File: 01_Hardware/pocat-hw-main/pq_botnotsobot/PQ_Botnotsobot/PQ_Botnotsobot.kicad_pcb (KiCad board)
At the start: 2 copper layers, 64 x 58 mm, 16 parts, among them J1 D2FLA, J2 D2FLA1

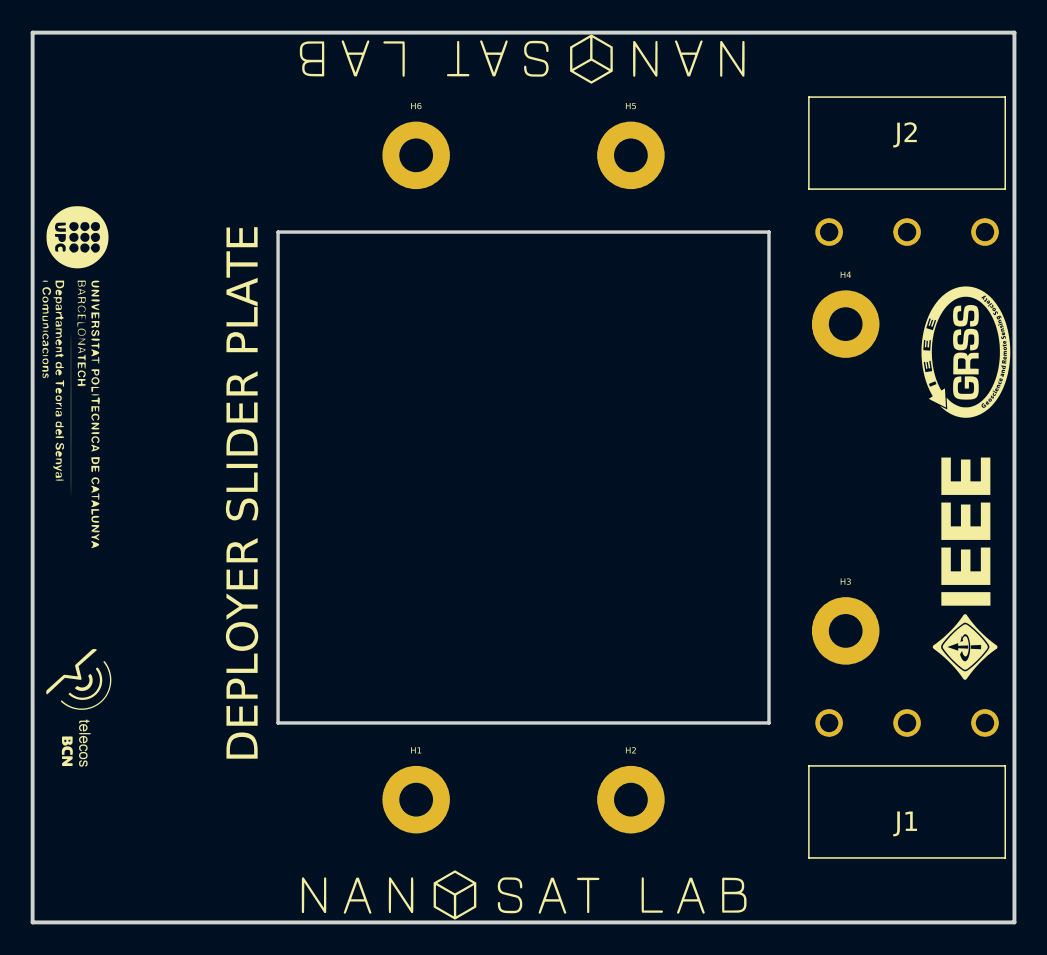
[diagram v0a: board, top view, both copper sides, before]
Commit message: Pcbs actualizados corregidos (son definitivos para mandarlos a fabricar con sus respectivos Gebers en una carpeta separada)
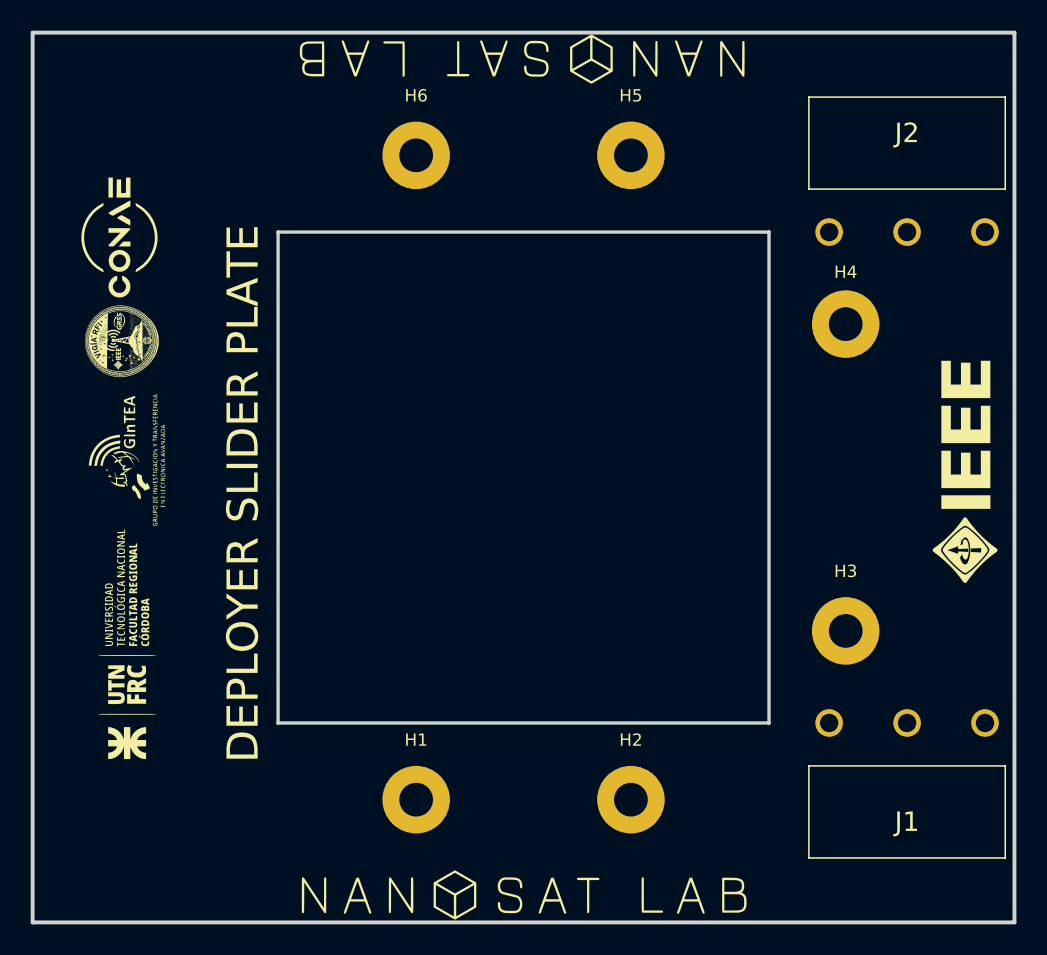
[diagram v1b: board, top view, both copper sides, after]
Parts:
- removed Annotation5: Silkscreen_Annotation, symbols-nsl:GRSS
- removed Annotation8: Silkscreen_Annotation, -nsl_symbols:UPC_positiu
- removed Annotation9: Silkscreen_Annotation, -nsl_symbols:Telecos
- added G***: LOGO, LOGO, F.Cu at (76.5, 53.4)
- added G***: LOGO, LOGO, F.Cu at (76.7, 61.1)
- added G***: LOGO, LOGO, F.Cu at (76.7, 73.1)
- added G***: LOGO, LOGO, F.Cu at (76.2, 46.6)
- moved Annotation6 6.31 mm to (131.4, 60.4)
